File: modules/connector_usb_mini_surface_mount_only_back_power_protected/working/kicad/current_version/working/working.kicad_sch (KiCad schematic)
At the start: 1 part, among them J1 scumnsmo

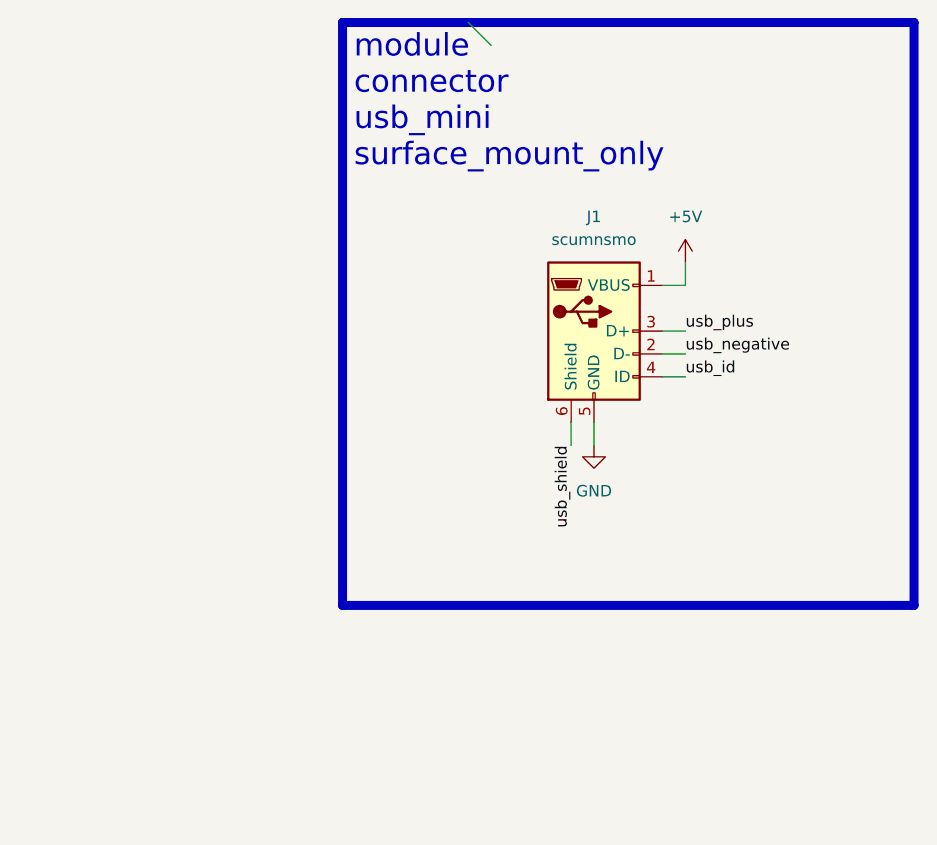
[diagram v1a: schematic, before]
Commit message: works.
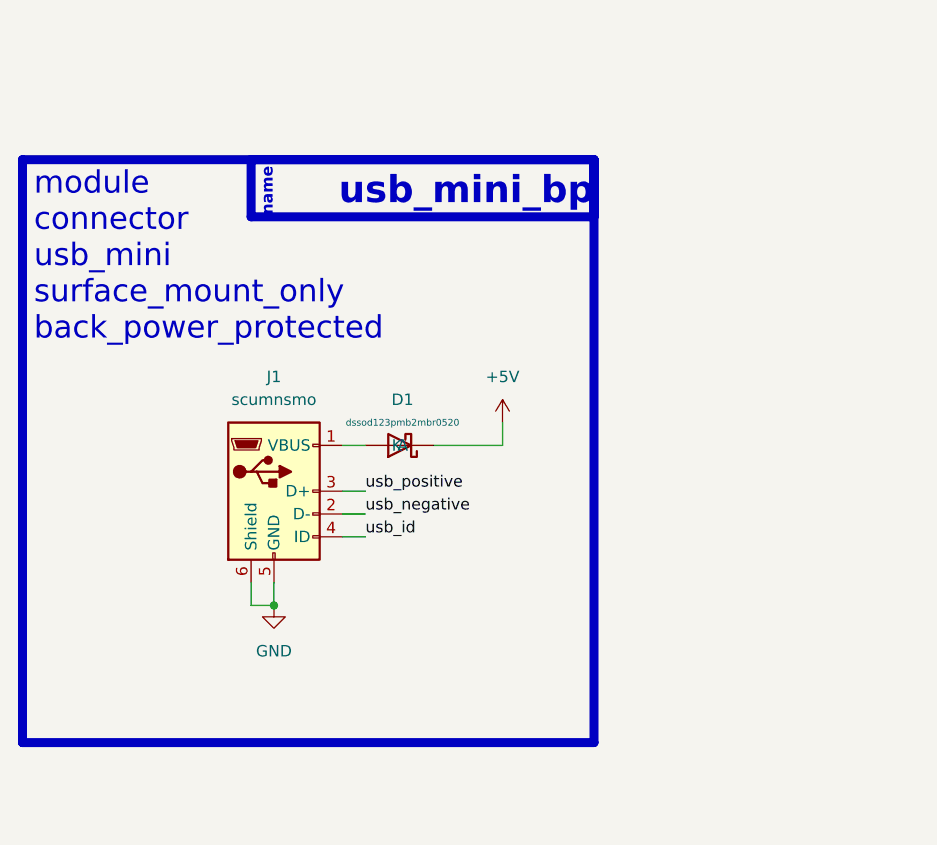
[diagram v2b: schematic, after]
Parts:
- added D1: dssod123pmb2mbr0520, oomlout_oomp_part_footprints:dssod123pmb2mbr0520_electronic_diode_schottky_sod_123_package_marking_b2_mbr0520, symbol oomlout_oomp_part_symbols:dssod123pmb2mbr0520_electronic_diode_schottky_sod_123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
- J1: footprint scumnsmo_electronic_socket_usb_mini_surface_mount_only -> oomlout_oomp_part_footprints:scumnsmo_electronic_socket_usb_mini_surface_mount_only
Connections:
- net usb_shield is gone; now on net GND: J1.6 (Shield)
- net +5V: now also D1.1 (K); no longer J1.1 (VBUS)
- net usb_plus renamed usb_positive
- new net: D1.2 (A), J1.1 (VBUS)
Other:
- note added: "module connector usb_mini surface_mount_only back_power_protected"
- note added: "name"
- note added: "usb_mini_bp"
- note removed: "module connector usb_mini surface_mount_only"
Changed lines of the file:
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@@
 (kicad_sch (version 20230121) (generator eeschema)
   (paper "A4")
-  (bus_entry (at 151.13 40.64) (size 2.54 2.54)
+  (junction (at 129.54 105.41) (diameter 0) (color 0 0 0 0)
+  )
+  (wire (pts (xy 129.54 102.87) (xy 129.54 105.41))
     (stroke (width 0) (type default))
   )
-  (wire (pts (xy 175.26 69.85) (xy 172.72 69.85))
+  (wire (pts (xy 137.16 87.63) (xy 139.7 87.63))
     (stroke (width 0) (type default))
   )
-  (wire (pts (xy 165.1 85.09) (xy 165.1 87.63))
+  (wire (pts (xy 137.16 97.79) (xy 139.7 97.79))
     (stroke (width 0) (type default))
   )
-  (wire (pts (xy 162.56 85.09) (xy 162.56 87.63))
+  (wire (pts (xy 137.16 95.25) (xy 139.7 95.25))
     (stroke (width 0) (type default))
   )
-  (wire (pts (xy 172.72 74.93) (xy 175.26 74.93))
+  (wire (pts (xy 154.94 85.09) (xy 154.94 87.63))
     (stroke (width 0) (type default))
   )
-  (wire (pts (xy 172.72 80.01) (xy 175.26 80.01))
+  (wire (pts (xy 154.94 87.63) (xy 147.32 87.63))
     (stroke (width 0) (type default))
   )
-  (wire (pts (xy 175.26 67.31) (xy 175.26 69.85))
+  (wire (pts (xy 127 105.41) (xy 129.54 105.41))
     (stroke (width 0) (type default))
   )
-  (wire (pts (xy 172.72 77.47) (xy 175.26 77.47))
+  (wire (pts (xy 127 102.87) (xy 127 105.41))
     (stroke (width 0) (type default))
   )
-  (rectangle (start 137.16 40.64) (end 200.66 105.41)
+  (wire (pts (xy 137.16 92.71) (xy 139.7 92.71))
+    (stroke (width 0) (type default))
+  )
+  (rectangle (start 127 55.88) (end 165.1 62.23)
+    (stroke (width 1) (type default))
+    (fill (type color) (color 0 0 0 0))
+  )
+  (rectangle (start 101.6 55.88) (end 165.1 120.65)
     (stroke (width 1) (type default))
     (fill (type none))
   )
-  (rectangle (start 199.39 97.79) (end 199.39 97.79)
-    (stroke (width 0) (type default))
-    (fill (type none))
+  (text "usb_mini_bp\n\n" (at 165.1 66.04 0)
+    (effects (font (size 3 3) (thickness 0.8) bold (color 255 255 255 1)) (justify right bottom))
   )
-  (text "module\nconnector\nusb_mini\nsurface_mount_only\n\n" (at 138.43 60.96 0)
+  (text "name" (at 129.54 62.23 90)
+    (effects (font (size 1.27 1.27) (thickness 0.254) bold (color 255 255 255 1)) (justify left bottom))
+  )
+  (text "module\nconnector\nusb_mini\nsurface_mount_only\nback_power_protected\n"
+    (at 102.87 76.2 0)
     (effects (font (size 2.5 2.5)) (justify left bottom))
   )
-  (label "usb_id" (at 175.26 80.01 0) (fields_autoplaced)
+  (label "usb_positive" (at 139.7 92.71 0) (fields_autoplaced)
     (effects (font (size 1.27 1.27)) (justify left bottom))
   )
-  (label "usb_plus" (at 175.26 74.93 0) (fields_autoplaced)
+  (label "usb_negative" (at 139.7 95.25 0) (fields_autoplaced)
     (effects (font (size 1.27 1.27)) (justify left bottom))
   )
-  (label "usb_negative" (at 175.26 77.47 0) (fields_autoplaced)
+  (label "usb_id" (at 139.7 97.79 0) (fields_autoplaced)
     (effects (font (size 1.27 1.27)) (justify left bottom))
   )
-  (label "usb_shield" (at 162.56 87.63 270) (fields_autoplaced)
-    (effects (font (size 1.27 1.27)) (justify right bottom))
-  )
-  (symbol (lib_id "oomlout_oomp_part_symbols:scumnsmo_electronic_socket_usb_mini_surface_mount_only") (at 165.1 74.93 0) (unit 1)
+  (symbol (lib_id "oomlout_oomp_part_symbols:dssod123pmb2mbr0520_electronic_diode_schottky_sod_123_package_marking_b2_mbr0520") (at 143.51 87.63 180) (unit 1)
     (in_bom yes) (on_board yes) (dnp no) (fields_autoplaced)
-    (property "Reference" "J1" (at 165.1 62.23 0)
+    (property "Reference" "D1" (at 143.8275 82.55 0)
       (effects (font (size 1.27 1.27)))
     )
-    (property "Value" "scumnsmo" (at 165.1 64.77 0)
+    (property "Value" "dssod123pmb2mbr0520" (at 143.8275 85.09 0)
+      (effects (font (size 0.75 0.75)))
+    )
+    (property "Footprint" "oomlout_oomp_part_footprints:dssod123pmb2mbr0520_electronic_diode_schottky_sod_123_package_marking_b2_mbr0520" (at 143.51 87.63 0)
+      (effects (font (size 1.27 1.27)) hide)
+    )
+    (property "Datasheet" "https://github.com/oomlout/oomlout_oomp_v3/parts/electronic_diode_schottky_sod_123_package_marking_b2_mbr0520/datasheet.pdf" (at 143.51 87.63 0)
+      (effects (font (size 1.27 1.27)) hide)
+    )
+    (pin "1")
+    (pin "2")
+    (instances
+      (project "working"
+        (path "/d7ac9d55-1973-40f4-b2a5-38a433b49fa0"
+          (reference "D1") (unit 1)
+        )
+      )
+    )
+  )
+  (symbol (lib_id "power:+5V") (at 154.94 85.09 0) (unit 1)
+    (in_bom yes) (on_board yes) (dnp no) (fields_autoplaced)
+    (property "Reference" "#PWR013" (at 154.94 88.9 0)
+      (effects (font (size 1.27 1.27)) hide)
+    )
+    (property "Value" "+5V" (at 154.94 80.01 0)
       (effects (font (size 1.27 1.27)))
     )
-    (property "Footprint" "scumnsmo_electronic_socket_usb_mini_surface_mount_only" (at 168.91 76.2 0)
+    (property "Footprint" "" (at 154.94 85.09 0)
       (effects (font (size 1.27 1.27)) hide)
     )
-    (property "Datasheet" "https://github.com/oomlout/oomlout_oomp_v3/parts/electronic_socket_usb_mini_surface_mount_only/datasheet.pdf" (at 168.91 76.2 0)
+    (property "Datasheet" "" (at 154.94 85.09 0)
+      (effects (font (size 1.27 1.27)) hide)
+    )
+    (pin "1")
+    (instances
+      (project "working"
+        (path "/5407c114-4107-4d84-8382-1717fb9d687c"
+          (reference "#PWR013") (unit 1)
+        )
+      )
+      (project "working"
+        (path "/d7ac9d55-1973-40f4-b2a5-38a433b49fa0"
+          (reference "#PWR02") (unit 1)
+        )
+      )
+    )
+  )
+  (symbol (lib_id "oomlout_oomp_part_symbols:scumnsmo_electronic_socket_usb_mini_surface_mount_only") (at 129.54 92.71 0) (unit 1)
+    (in_bom yes) (on_board yes) (dnp no) (fields_autoplaced)
+    (property "Reference" "J1" (at 129.54 80.01 0)
+      (effects (font (size 1.27 1.27)))
+    )
+    (property "Value" "scumnsmo" (at 129.54 82.55 0)
+      (effects (font (size 1.27 1.27)))
+    )
+    (property "Footprint" "oomlout_oomp_part_footprints:scumnsmo_electronic_socket_usb_mini_surface_mount_only" (at 133.35 93.98 0)
+      (effects (font (size 1.27 1.27)) hide)
+    )
+    (property "Datasheet" "https://github.com/oomlout/oomlout_oomp_v3/parts/electronic_socket_usb_mini_surface_mount_only/datasheet.pdf" (at 133.35 93.98 0)
       (effects (font (size 1.27 1.27)) hide)
     )
@@
     )
   )
-  (symbol (lib_id "power:+5V") (at 175.26 67.31 0) (unit 1)
+  (symbol (lib_id "power:GND") (at 129.54 105.41 0) (unit 1)
     (in_bom yes) (on_board yes) (dnp no) (fields_autoplaced)
-    (property "Reference" "#PWR04" (at 175.26 71.12 0)
+    (property "Reference" "#PWR012" (at 129.54 111.76 0)
       (effects (font (size 1.27 1.27)) hide)
     )
-    (property "Value" "+5V" (at 175.26 62.23 0)
+    (property "Value" "GND" (at 129.54 110.49 0)
       (effects (font (size 1.27 1.27)))
     )
-    (property "Footprint" "" (at 175.26 67.31 0)
+    (property "Footprint" "" (at 129.54 105.41 0)
       (effects (font (size 1.27 1.27)) hide)
     )
-    (property "Datasheet" "" (at 175.26 67.31 0)
+    (property "Datasheet" "" (at 129.54 105.41 0)
       (effects (font (size 1.27 1.27)) hide)
     )
@@
     (instances
       (project "working"
-        (path "/d7ac9d55-1973-40f4-b2a5-38a433b49fa0"
-          (reference "#PWR04") (unit 1)
+        (path "/5407c114-4107-4d84-8382-1717fb9d687c"
+          (reference "#PWR012") (unit 1)
         )
       )
-    )
-  )
-  (symbol (lib_id "power:GND") (at 165.1 87.63 0) (unit 1)
-    (in_bom yes) (on_board yes) (dnp no) (fields_autoplaced)
-    (property "Reference" "#PWR03" (at 165.1 93.98 0)
-      (effects (font (size 1.27 1.27)) hide)
-    )
-    (property "Value" "GND" (at 165.1 92.71 0)
-      (effects (font (size 1.27 1.27)))
-    )
-    (property "Footprint" "" (at 165.1 87.63 0)
-      (effects (font (size 1.27 1.27)) hide)
-    )
-    (property "Datasheet" "" (at 165.1 87.63 0)
-      (effects (font (size 1.27 1.27)) hide)
-    )
-    (pin "1")
-    (instances
       (project "working"
         (path "/d7ac9d55-1973-40f4-b2a5-38a433b49fa0"
-          (reference "#PWR03") (unit 1)
+          (reference "#PWR01") (unit 1)
         )
       )
